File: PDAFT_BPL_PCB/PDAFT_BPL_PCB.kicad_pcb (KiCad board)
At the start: 2 copper layers, 63.4 x 85.5 mm, 19 parts

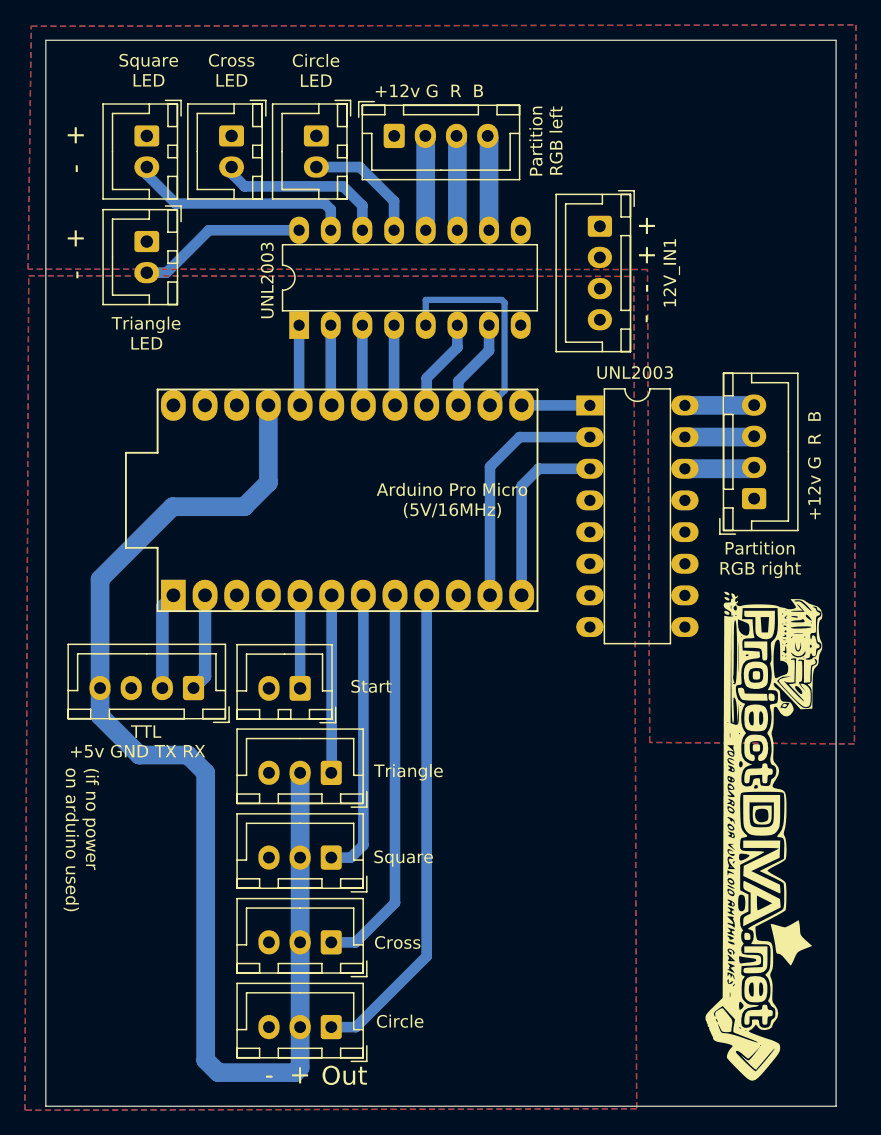
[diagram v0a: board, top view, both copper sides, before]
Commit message: board update
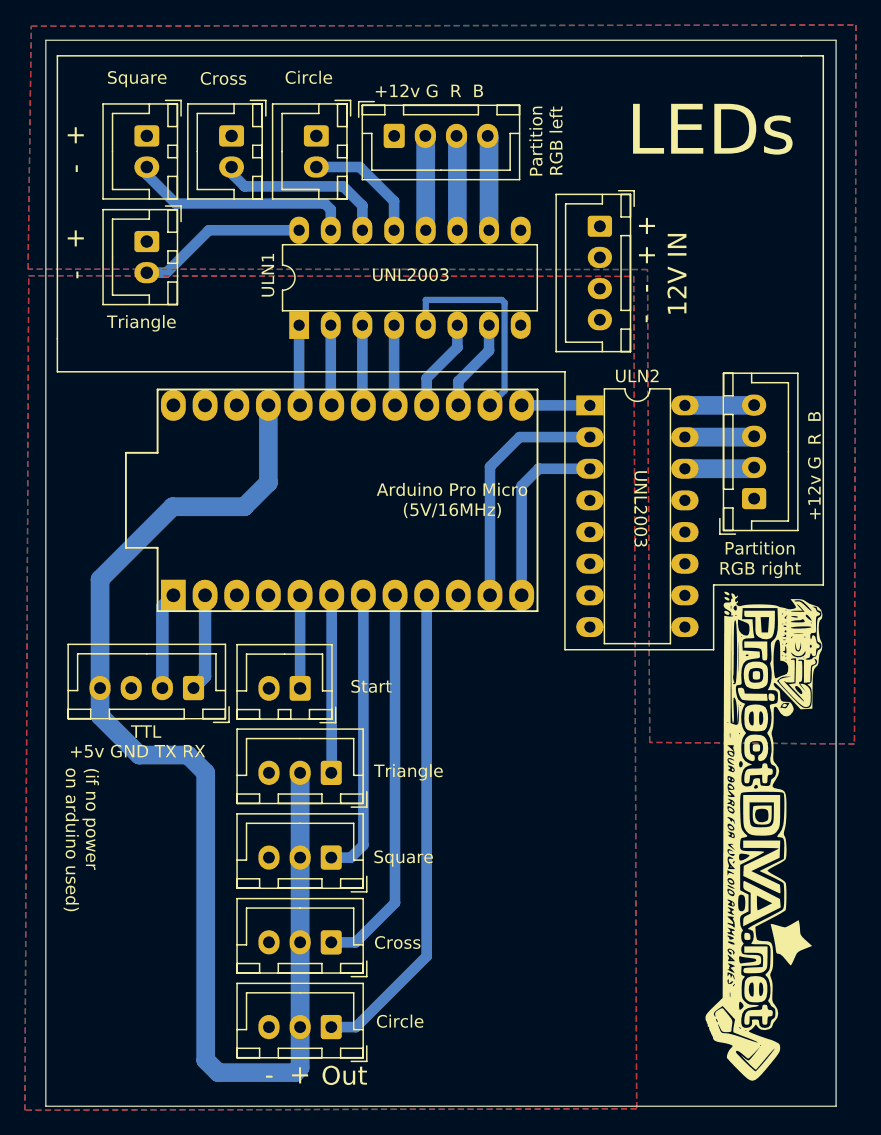
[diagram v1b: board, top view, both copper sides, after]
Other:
- board text added: "LEDs"
